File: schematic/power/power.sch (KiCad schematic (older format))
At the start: 29 parts

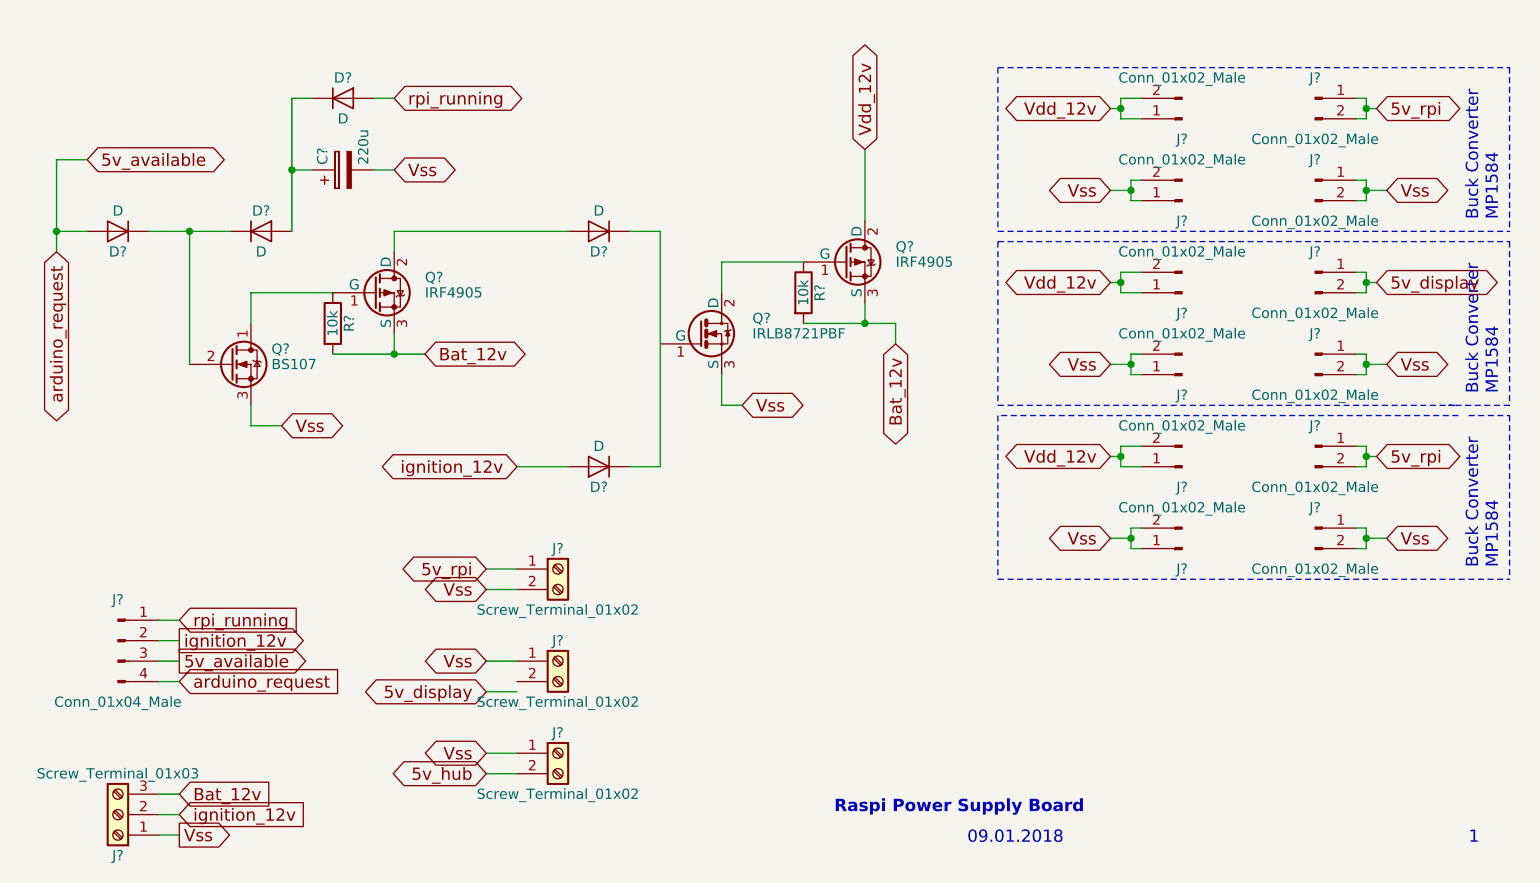
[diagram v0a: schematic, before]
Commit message: ok, lets go again
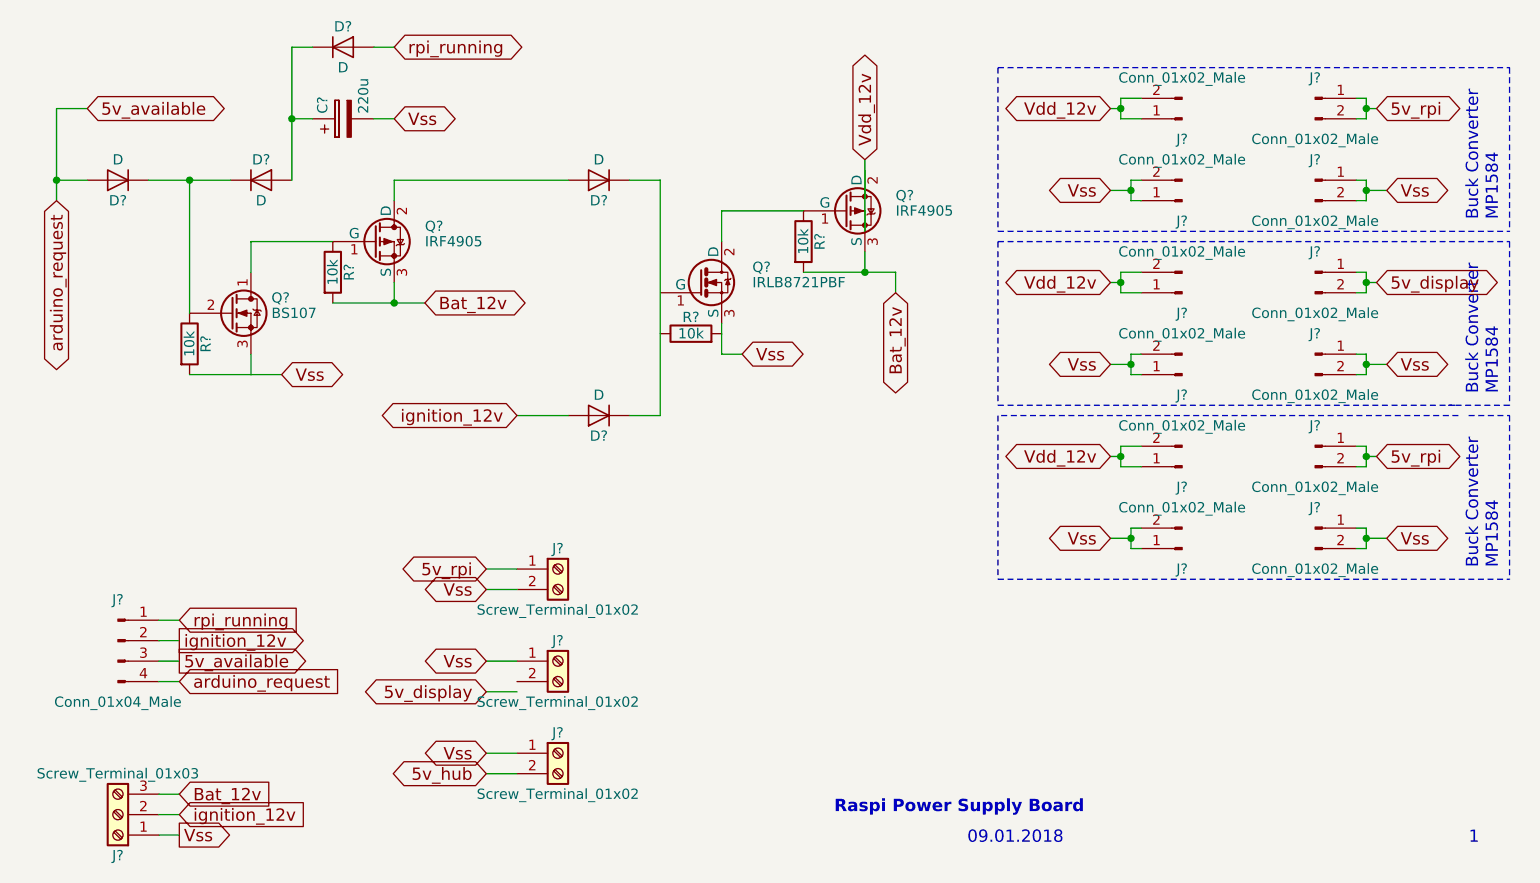
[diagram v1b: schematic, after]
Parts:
- added R? (x2): 10k, symbol R
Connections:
- wire segments 108 -> 91
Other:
- moved on the sheet: C?, D?, Q?, R?
